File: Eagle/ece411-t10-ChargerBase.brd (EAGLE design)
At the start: 44.6 x 80.3 mm, 51 parts, among them IC1 NE5532D, IC2 TINY24/44/84-SSU, IC3 NE5532D, IC5 AZ1117IH-5.0V, Q1 2N3906, T1 2N3904, T2 2N3904, T3 2N3904

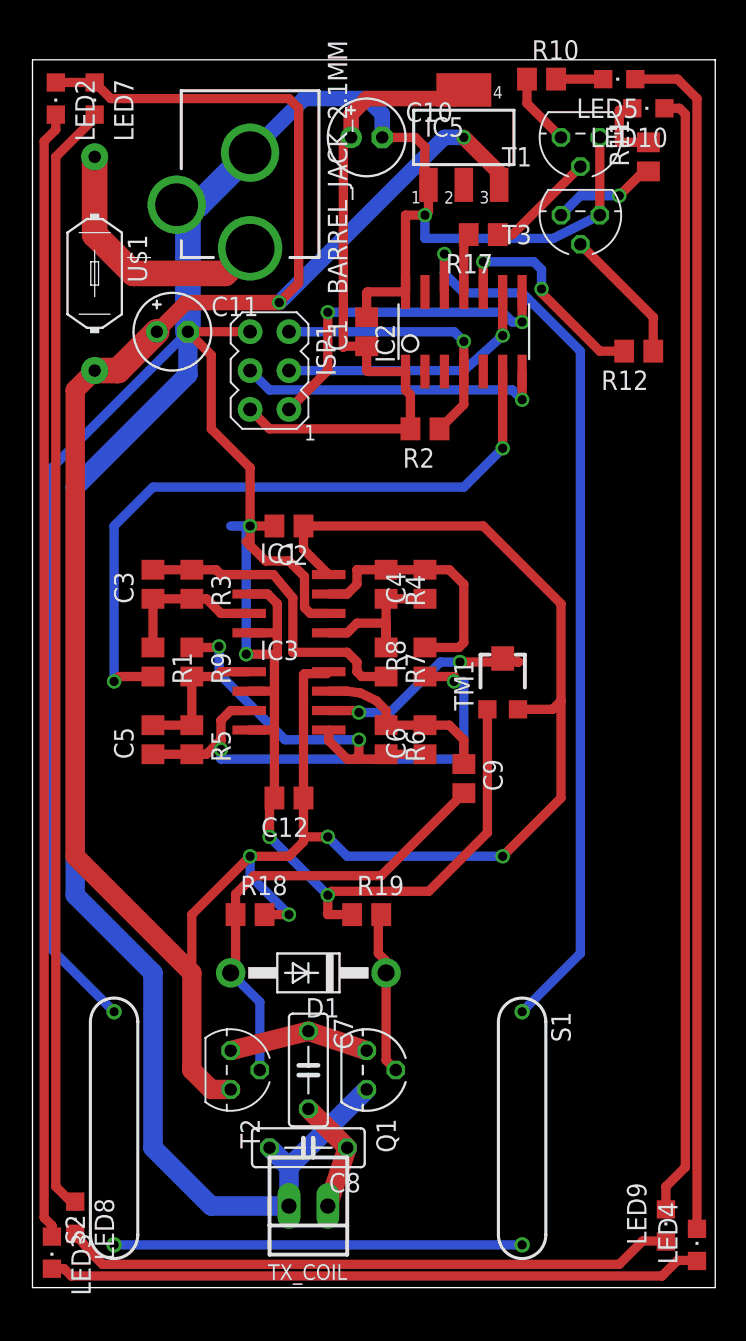
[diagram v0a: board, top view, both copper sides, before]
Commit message: Boards + schematics rev2
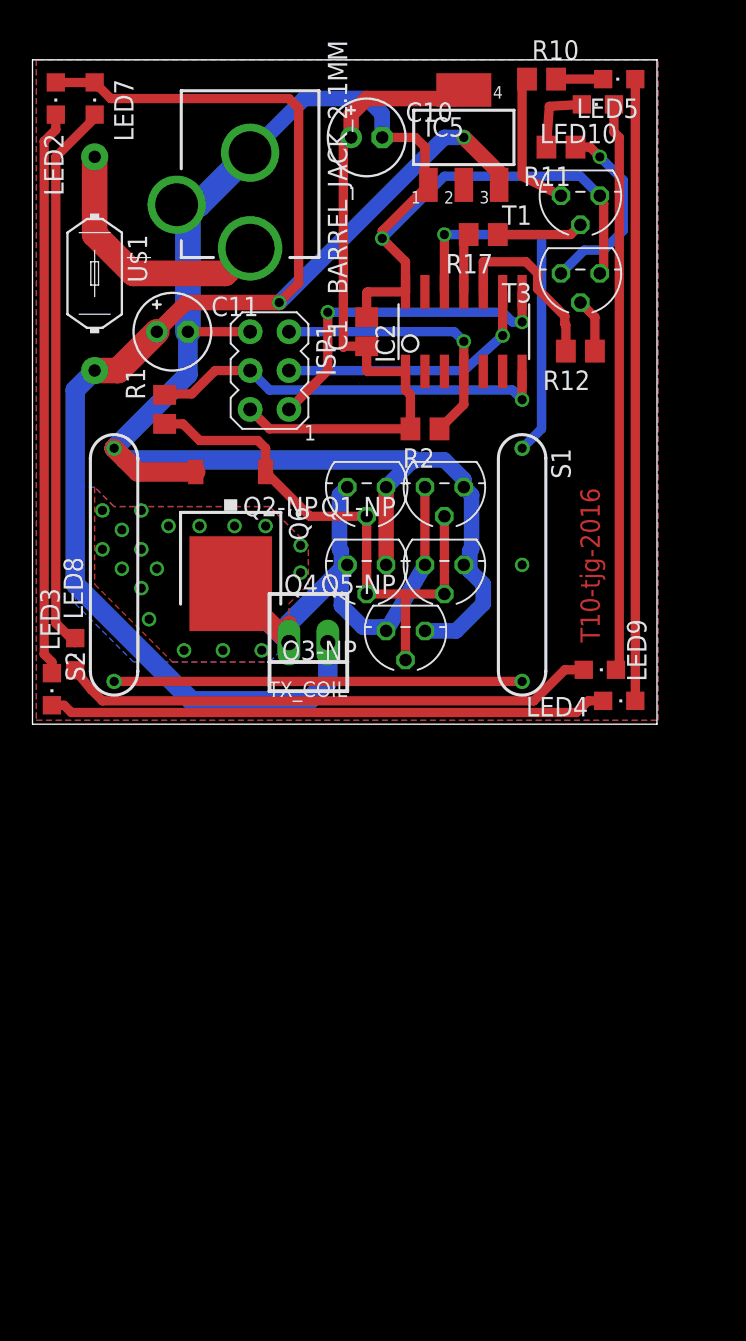
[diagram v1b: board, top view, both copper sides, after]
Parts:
- removed C12, C2, C9: 100n, rcl:C0805
- removed C3, C4, C5, C6: 1nF, rcl:C0805
- removed C7: 1uF, adafruit:C050-025X075
- removed C8: 10nF, adafruit:C050-025X075
- removed D1: 1N4004, adafruit:DO41-10
- removed IC1, IC3: NE5532D, linear:SO08
- removed Q1: 2N3906, transistor-pnp:TO92
- removed R18, R19: 10k, rcl:R0805
- removed R3, R4, R5, R6, R7, R8, R9: 1k, rcl:R0805
- removed T2: 2N3904, transistor:TO92
- removed TM1: 100k, adafruit:TC33X
- added Q1-NP, Q2-NP, Q3-NP, Q4, Q5-NP: NP, transistor-fet:TO-92
- added Q6: RFD16N05LSM9ACTTO252, _VMS:TO252
- R1: value 1k -> 0R
- R12, R17: value 1k -> 5k
- S1, S2: value REED-SWITCH-MK6-6 -> REED-SWITCH
- moved LED8 36.8 mm to (2.54, 41.1)
- moved LED3 36.8 mm to (1.02, 38.9)
- moved S1 36.8 mm to (31.8, 47.0)
- moved S2 36.8 mm to (5.08, 47.0)
- moved TX_COIL 36.8 mm to (17.8, 41.9)
- moved LED9 36.6 mm to (36.8, 40.1), turned to 270 degrees
- moved LED4 35.9 mm to (38.1, 38.1), turned to 270 degrees
- moved R1 16.5 mm to (8.38, 57.1), turned to 90 degrees
- moved R11 5.75 mm to (34.3, 74.3), turned to 180 degrees
- moved T1 3.81 mm to (35.6, 71.1)
- moved R12 3.81 mm to (35.6, 61.0)
- moved T3 3.81 mm to (35.6, 66.0)
- moved LED10 3.31 mm to (36.7, 77.1)
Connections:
- removed net COIL_DRIVER: C6.2, C9.1, IC3.7, R6.1
- removed net N$1: C3.1, IC1.3, R1.1, R3.2
- removed net N$10: C4.2, IC1.7, R4.1, R8.2
- removed net N$11: C5.1, IC3.3, R5.2, R8.1
- removed net N$12: C5.2, IC3.1, R5.1, R9.2
- removed net N$13: C6.1, IC3.5, R6.2, R9.1
- removed net N$15: IC3.6, TM1.2
- removed net N$27: C7.1, Q1.3, T2.3
- removed net N$28: C9.2, D1.A, R18.1, T2.2
- removed net N$29: D1.C, Q1.2, R19.2
- removed net N$30: C7.2, C8.1, TX_COIL.1
- removed net N$8: C3.2, IC1.1, R3.1, R7.2
- removed net N$9: C4.1, IC1.5, R4.2, R7.1
- new net DRAIN: Q1-NP.3, Q2-NP.3, Q3-NP.3, Q4.3, Q5-NP.3, Q6.3, TX_COIL.2
- net GND: now also Q1-NP.1, Q2-NP.1, Q3-NP.1, Q4.1, Q5-NP.1, Q6.2; no longer C12.2, C2.2, C8.2, IC1.2, IC1.4, IC1.6, IC3.2, IC3.4, Q1.1, R19.1, TM1.1, TX_COIL.2
- net MOSI: now also R1.2
- net PWM: now also Q1-NP.2, Q2-NP.2, Q3-NP.2, Q4.2, Q5-NP.2, Q6.1, R1.1; no longer IC2.6, R1.2
- net VDD: now also TX_COIL.1; no longer C12.1, C2.1, IC1.8, IC3.8, R18.2, T2.1, TM1.3
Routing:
- net GND: track 286.7 -> 132.4 mm, vias 5 -> 2
- net VDD: track 208.1 -> 103.2 mm, vias 6 -> 2
- net N$20: track 78.4 -> 40.6 mm
- net N$24: track 73.2 -> 36.4 mm
- net N$18: track 73.9 -> 37.0 mm
- net N$26: track 73.6 -> 37.2 mm
- net DRAIN: track 0.00 -> 36.1 mm, vias 0 -> 18
- net PIN12: track 59.5 -> 24.6 mm
- net N$11: track 33.3 -> 0.00 mm, vias 2 -> 0
- net N$28: track 30.1 -> 0.00 mm
- net N$13: track 23.5 -> 0.00 mm, vias 2 -> 0
- net N$8: track 20.7 -> 0.00 mm
- net N$10: track 16.9 -> 0.00 mm
- net N$15: track 14.9 -> 0.00 mm, vias 2 -> 0
- net COIL_DRIVER: track 12.2 -> 0.00 mm
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- added copper zone on layer 1, net DRAIN
- added copper zone on layer 16, net DRAIN
- added copper zone on layer 1, net GND
- added copper zone on layer 16, net GND
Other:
- board size 44.6 x 80.3 mm -> 40.8 x 43.4 mm
- board text added: "T10-tjg-2016"
